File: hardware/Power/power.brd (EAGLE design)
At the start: 70 x 70 mm, 44 parts, among them IC10 ACS712ELCTR-05B-T, IC20 LM358_SOIC, K1 SSR, Q1 PNP, T20 ZMPT101B, U4 PC817XI, X1 057-006-1

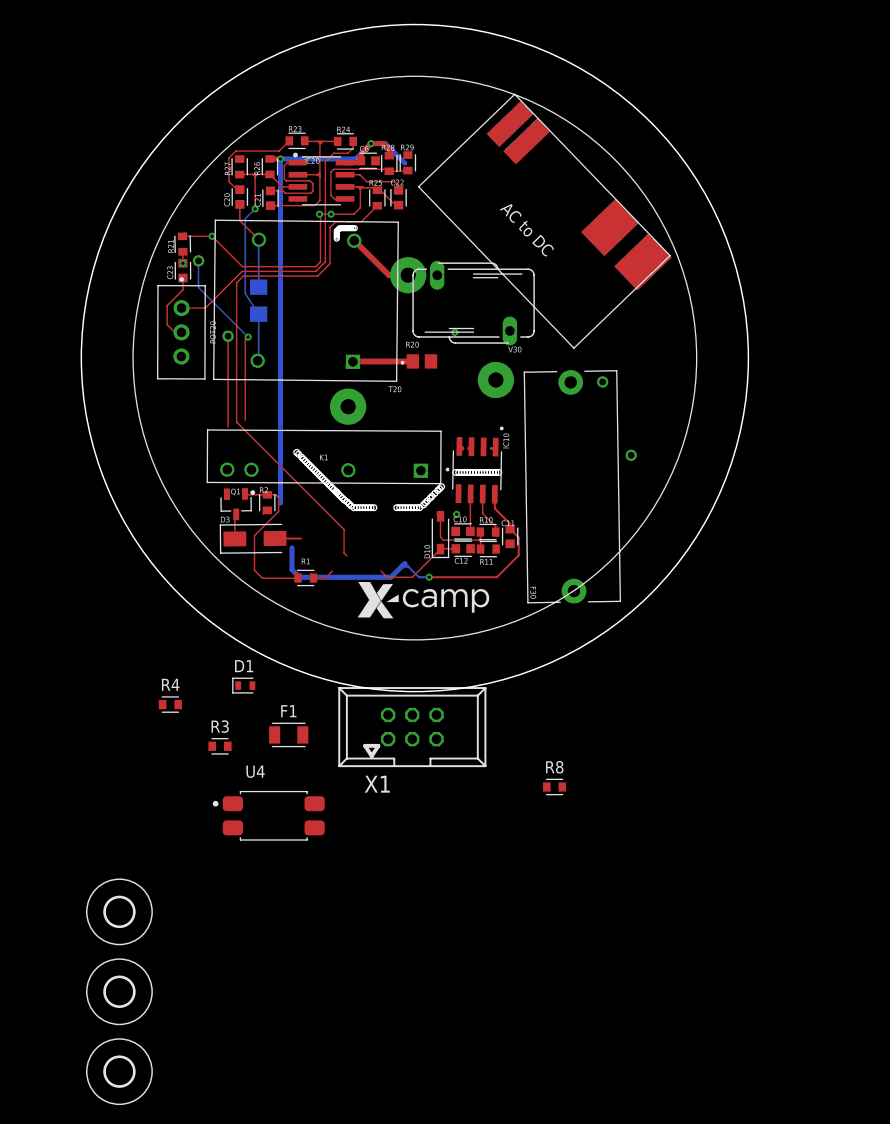
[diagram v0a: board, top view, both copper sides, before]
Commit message: bakcup before ganti ukuran smd
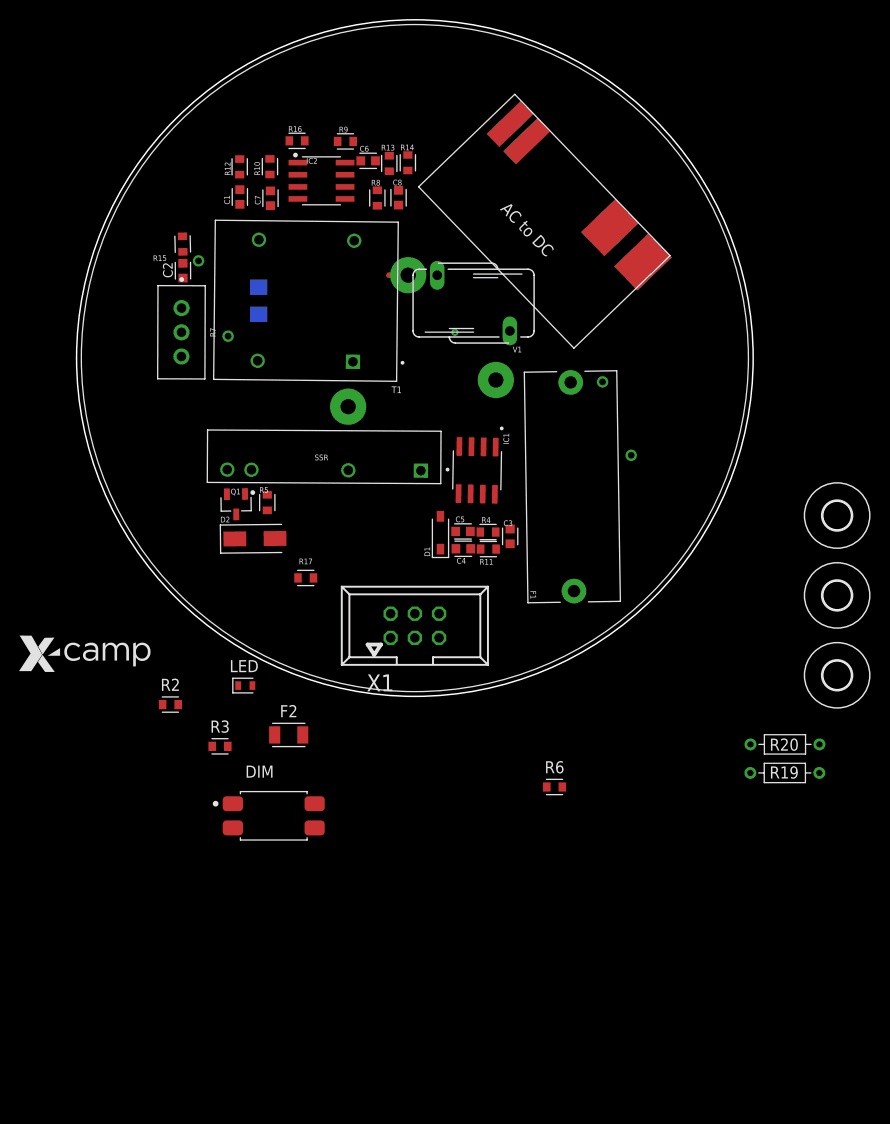
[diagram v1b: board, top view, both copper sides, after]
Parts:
- removed D10: 1N4448W, Diode:SOD3715X135
- removed F30: 4527, Fuse Holder:4527
- removed R22: 100, rcl:R1206
- removed R25: 100K, Resistor:RESC1608X60
- removed R26: 10k, Resistor:RESC1608X60
- added F2: FUSE PTC 1A, Circuit-Protection:FUSC3215X82N
- added LED: LED_BLUE, LED:LEDC1608X55N_FLAT-B
- added R17: 10K, Resistor:RESC1608X60
- added R19: 330K, Resistor:RESAD724W46L381D178B
- added R5, R6: 4.7K, Resistor:RESC1608X60
- AC-DC: value HI-LINKVERTICAL -> (none)
- D1: value LED_BLUE -> 1N4448W; device LED:LEDC1608X55N_FLAT-B -> Diode:SOD3715X135
- F1: value FUSE PTC 1A -> HOLDER 5x20; device Circuit-Protection:FUSC3215X82N -> Fuse Holder:4527
- R1: value 10k -> 100; device Resistor:RESC1608X60 -> rcl:R1206
- R10: value 2k -> 10K
- R11, R12, R13, R14, R15, R16: value 10k -> 10K
- R2: value 4.7k -> 330
- R20: value 820K -> 330K; device rcl:R0805 -> Resistor:RESAD724W46L381D178B
- R4: value 330 -> 2k
- R7: value 10K -> 100K
- R8: value 4.7k -> 100K
- moved H1 86.0 mm to (44.3, -16.5)
- moved H2 86.0 mm to (44.3, -24.9)
- moved H3 86.0 mm to (44.3, -33.3)
- moved R8 64.5 mm to (-3.94, 16.8), turned to 270 degrees
- moved R20 55.4 mm to (38.8, -40.5)
- moved R10 44.6 mm to (-15.2, 20.1), turned to 90 degrees
- moved F1 39.5 mm to (16.5, -13.5), turned to 90.9 degrees
- moved R4 37.9 mm to (7.68, -18.3), turned to 180 degrees
- moved R1 29.5 mm to (-16.4, 6.02), flipped to the bottom, turned to 270 degrees
- moved D1 26.0 mm to (2.69, -18.3), turned to 90 degrees
- moved R2 23.5 mm to (-25.7, -36.4), turned to 0 degrees
- moved X1 10.6 mm to (0.00, -28.1)
- renumbered C10 to C5, C11 to C3, C12 to C4, C20 to C1, C21 to C7, C22 to C8, C23 to C2, D3 to D2, IC10 to IC1, IC20 to IC2, K1 to SSR, POT20 to R7, PS1 to AC-DC, R21 to R15, R23 to R16, R24 to R9, R27 to R12, R28 to R13, R29 to R14, T20 to T1, U4 to DIM, V30 to V1
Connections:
- new net N$5: R19.2, R20.1
- net 5V: now also F2.2, R10.2; no longer F1.2, R26.2
- net ADC_CURRENT: now also D1.1; no longer D10.1
- net ADC_VOLTAGE: now also R8.2; no longer R25.2
- net GND: now also LED.C; no longer D1.C
- net IO_RELAY: now also R17.2, R6.1; no longer R1.2, R8.1
- net L: now also F1.1; no longer F30.1
- net L_FUSE: now also F1.2, R19.1; no longer F30.2, R20.2
- net L_ZMPT: now also R20.2; no longer R20.1
- net N$1: now also R1.1; no longer R22.1
- net N$12: now also R5.2; no longer R2.2
- net N$13: now also R17.1, R5.1; no longer R1.1, R2.1
- net N$16: now also R8.1; no longer R25.1
- net N$22: now also F2.1; no longer F1.1
- net N$24: now also LED.A; no longer D1.A
- net N$27: now also R2.1; no longer R4.1
- net N$4: now also R4.1; no longer R10.1
- net N$9: now also D1.2, R4.2; no longer D10.2, R10.2
- net POS-A: now also R1.2, R10.1; no longer R22.2, R26.1
- net PWM_DIM: now also R2.2; no longer R4.2
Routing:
- net 5V: track 98.4 -> 0.00 mm, vias 3 -> 0
- net ADC_VOLTAGE: track 53.8 -> 0.00 mm
- net N$16: track 35.0 -> 0.00 mm, vias 3 -> 0
- net OUT-A: track 31.8 -> 0.00 mm
- net POS-A: track 27.8 -> 0.00 mm, vias 1 -> 0
- net DIM-: track 19.0 -> 0.00 mm, vias 1 -> 0
- net N$8: track 18.9 -> 0.00 mm
- net N$13: track 17.2 -> 0.00 mm
- net POS-B: track 12.4 -> 0.00 mm
- net N$2: track 11.6 -> 0.00 mm
- net N$3: track 11.0 -> 0.00 mm
- net N$1: track 9.53 -> 0.00 mm
- net DIM+: track 9.52 -> 0.00 mm
- net ADC_CURRENT: track 9.40 -> 0.00 mm
- net N$9: track 8.88 -> 0.00 mm
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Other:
- board size 70 x 70 mm -> 71 x 71 mm
